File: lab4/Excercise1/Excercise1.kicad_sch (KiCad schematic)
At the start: 6 parts, among them SW1 SW_SPDT

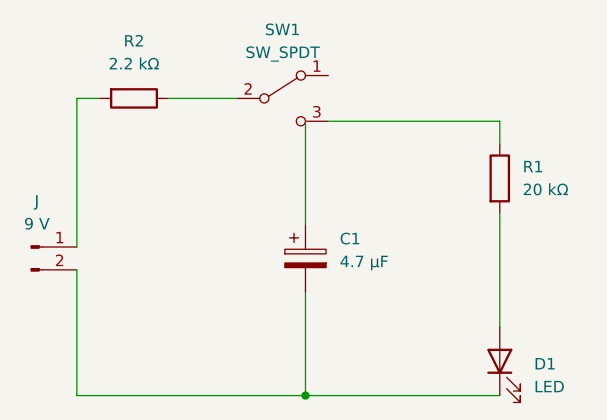
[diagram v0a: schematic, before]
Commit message: Update Exercise 1
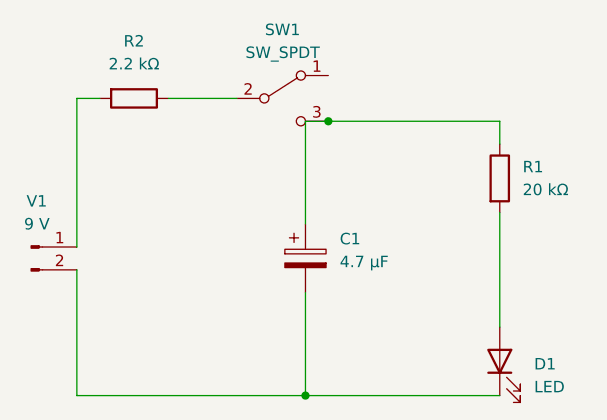
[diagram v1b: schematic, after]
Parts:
- C1: footprint (none) -> Capacitor_THT:C_Radial_D5.0mm_H5.0mm_P2.00mm
- D1: footprint (none) -> LED_THT:LED_D5.0mm
- R1, R2: footprint (none) -> Resistor_THT:R_Axial_DIN0516_L15.5mm_D5.0mm_P20.32mm_Horizontal
- SW1: footprint (none) -> Button_Switch_THT:SW_E-Switch_EG1224_SPDT_Angled
- V1: renamed from J; footprint (none) -> Connector_JST:JST_PH_B2B-PH-K_1x02_P2.00mm_Vertical
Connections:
- net at C1.1: now also R1.1, SW1.3 (C)
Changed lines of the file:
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@@
   (junction (at 148.59 116.84) (diameter 0) (color 0 0 0 0)
+  )
+  (junction (at 151.13 86.36) (diameter 0) (color 0 0 0 0)
   )
   (wire (pts (xy 123.19 102.87) (xy 123.19 116.84))
@@
     (stroke (width 0) (type default) (color 0 0 0 0))
   )
-  (wire (pts (xy 148.59 86.36) (xy 148.59 97.79))
+  (wire (pts (xy 148.59 86.36) (xy 151.13 86.36))
     (stroke (width 0) (type default) (color 0 0 0 0))
   )
@@
     (stroke (width 0) (type default) (color 0 0 0 0))
   )
+  (wire (pts (xy 148.59 97.79) (xy 148.59 86.36))
+    (stroke (width 0) (type default) (color 0 0 0 0))
+  )
   (wire (pts (xy 123.19 83.82) (xy 123.19 100.33))
     (stroke (width 0) (type default) (color 0 0 0 0))
@@
       (effects (font (size 1.27 1.27)) (justify right))
     )
-    (property "Footprint" "" (id 2) (at 170.18 113.03 0)
+    (property "Footprint" "LED_THT:LED_D5.0mm" (id 2) (at 170.18 113.03 0)
       (effects (font (size 1.27 1.27)) hide)
     )
@@
     (property "Reference" "R2" (id 0) (at 129.54 77.47 90))
     (property "Value" "2.2 kΩ" (id 1) (at 129.54 80.01 90))
-    (property "Footprint" "" (id 2) (at 129.54 82.042 90)
+    (property "Footprint" "Resistor_THT:R_Axial_DIN0516_L15.5mm_D5.0mm_P20.32mm_Horizontal" (id 2) (at 129.54 82.042 90)
       (effects (font (size 1.27 1.27)) hide)
     )
@@
       (effects (font (size 1.27 1.27)) (justify left))
     )
-    (property "Footprint" "" (id 2) (at 149.5552 105.41 0)
+    (property "Footprint" "Capacitor_THT:C_Radial_D5.0mm_H5.0mm_P2.00mm" (id 2) (at 149.5552 105.41 0)
       (effects (font (size 1.27 1.27)) hide)
     )
@@
     (property "Reference" "SW1" (id 0) (at 146.05 76.2 0))
     (property "Value" "SW_SPDT" (id 1) (at 146.05 78.74 0))
-    (property "Footprint" "" (id 2) (at 146.05 83.82 0)
+    (property "Footprint" "Button_Switch_THT:SW_E-Switch_EG1224_SPDT_Angled" (id 2) (at 146.05 83.82 0)
       (effects (font (size 1.27 1.27)) hide)
     )
@@
       (effects (font (size 1.27 1.27)) (justify left))
     )
-    (property "Footprint" "" (id 2) (at 168.402 92.71 90)
+    (property "Footprint" "Resistor_THT:R_Axial_DIN0516_L15.5mm_D5.0mm_P20.32mm_Horizontal" (id 2) (at 168.402 92.71 90)
       (effects (font (size 1.27 1.27)) hide)
     )
@@
   (symbol (lib_id "Connector:Conn_01x02_Male") (at 118.11 100.33 0) (unit 1)
     (in_bom yes) (on_board yes) (fields_autoplaced)
-    (property "Reference" "J" (id 0) (at 118.745 95.25 0))
+    (property "Reference" "V1" (id 0) (at 118.745 95.25 0))
     (property "Value" "9 V" (id 1) (at 118.745 97.79 0))
-    (property "Footprint" "" (id 2) (at 118.11 100.33 0)
+    (property "Footprint" "Connector_JST:JST_PH_B2B-PH-K_1x02_P2.00mm_Vertical" (id 2) (at 118.11 100.33 0)
       (effects (font (size 1.27 1.27)) hide)
     )
@@
   (symbol_instances
     (path "/3539fdc4-3667-4af4-8a0f-e98327ef01a5"
-      (reference "C1") (unit 1) (value "4.7 μF") (footprint "")
+      (reference "C1") (unit 1) (value "4.7 μF") (footprint "Capacitor_THT:C_Radial_D5.0mm_H5.0mm_P2.00mm")
     )
     (path "/1cb91c99-c531-411d-a595-ed15c35ebdff"
-      (reference "D1") (unit 1) (value "LED") (footprint "")
+      (reference "D1") (unit 1) (value "LED") (footprint "LED_THT:LED_D5.0mm")
+    )
+    (path "/d9cc5002-8438-4d2b-aab0-57ff494235ae"
+      (reference "R1") (unit 1) (value "20 kΩ") (footprint "Resistor_THT:R_Axial_DIN0516_L15.5mm_D5.0mm_P20.32mm_Horizontal")
+    )
+    (path "/22ba558d-a624-4de4-8bef-7e6faf4b6c89"
+      (reference "R2") (unit 1) (value "2.2 kΩ") (footprint "Resistor_THT:R_Axial_DIN0516_L15.5mm_D5.0mm_P20.32mm_Horizontal")
+    )
+    (path "/5563cd8f-ac6f-4d3a-af0f-b2e96dd62364"
+      (reference "SW1") (unit 1) (value "SW_SPDT") (footprint "Button_Switch_THT:SW_E-Switch_EG1224_SPDT_Angled")
     )
     (path "/fefeb908-eb8d-4755-83e1-d2105858d703"
-      (reference "J") (unit 1) (value "9 V") (footprint "")
-    )
-    (path "/d9cc5002-8438-4d2b-aab0-57ff494235ae"
-      (reference "R1") (unit 1) (value "20 kΩ") (footprint "")
-    )
-    (path "/22ba558d-a624-4de4-8bef-7e6faf4b6c89"
-      (reference "R2") (unit 1) (value "2.2 kΩ") (footprint "")
-    )
-    (path "/5563cd8f-ac6f-4d3a-af0f-b2e96dd62364"
-      (reference "SW1") (unit 1) (value "SW_SPDT") (footprint "")
+      (reference "V1") (unit 1) (value "9 V") (footprint "Connector_JST:JST_PH_B2B-PH-K_1x02_P2.00mm_Vertical")
     )
   )
